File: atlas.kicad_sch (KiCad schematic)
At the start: 26 parts, among them J1 AudioJack3, J2 Micro_SD_Card, SW1 SW_Push, SW2 SW_SPST, SW3 SW_Push, SW4 SW_Push, SW5 SW_Push, SW6 SW_Push, U1 ATmega328-P, U2 DAC8571IDGK, U3 Nokia_5110_LCD, U4 NE5532, Y1 Crystal

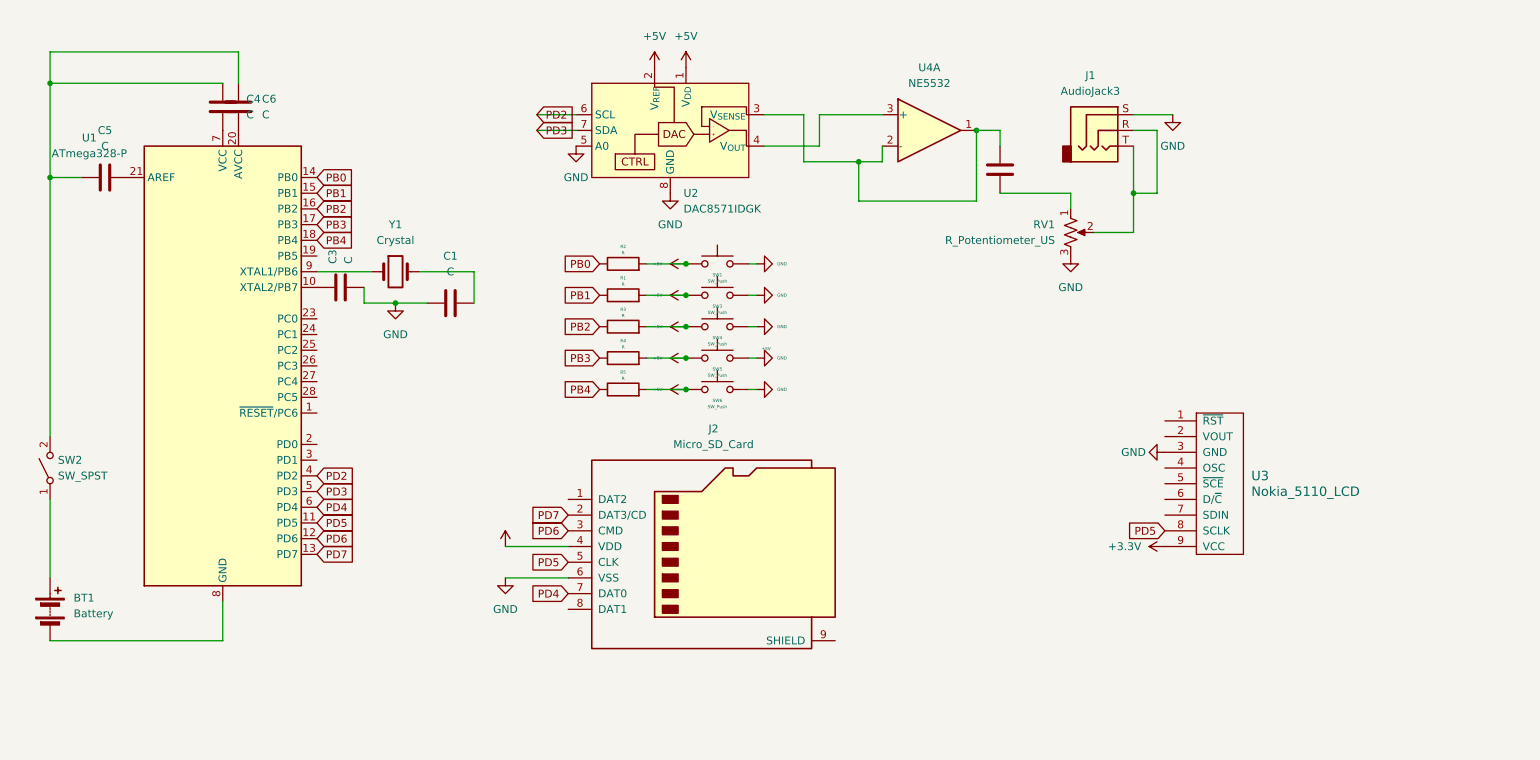
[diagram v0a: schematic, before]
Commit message: Add files via upload
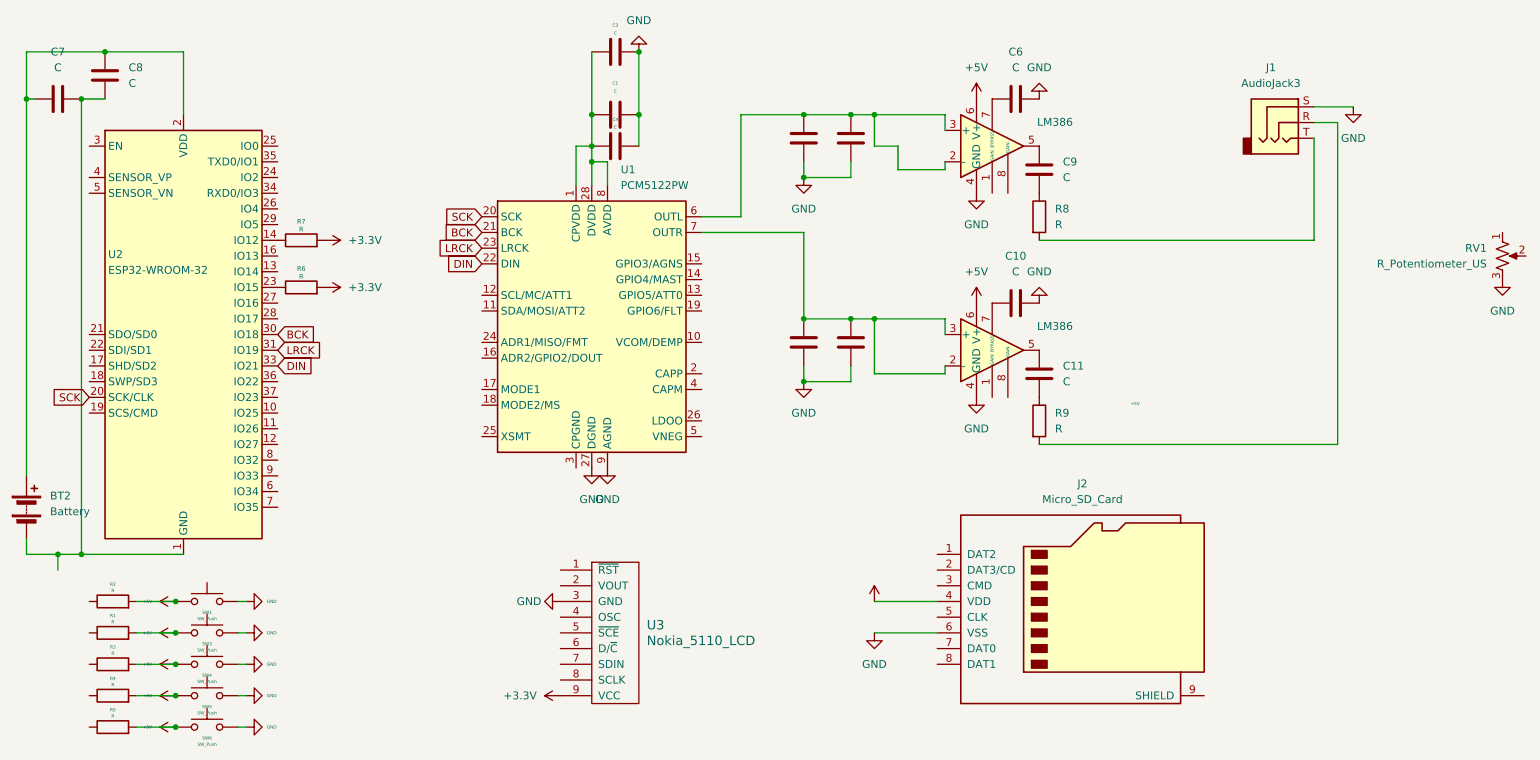
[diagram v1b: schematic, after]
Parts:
- removed BT1: Battery, symbol Device:Battery
- removed SW2: SW_SPST, Button_Switch_THT:SW_PUSH_6mm, symbol Switch:SW_SPST
- removed U1: ATmega328-P, Package_DFN_QFN:HVQFN-32-1EP_5x5mm_P0.5mm_EP3.1x3.1mm, symbol MCU_Microchip_ATmega:ATmega328-P
- removed U2: DAC8571IDGK, Package_SO:MSOP-8_3x3mm_P0.65mm, symbol Analog_DAC:DAC8571IDGK
- removed U4: NE5532, Package_CSP:LFCSP-8_2x2mm_P0.5mm, symbol Amplifier_Operational:NE5532
- removed Y1: Crystal, Crystal:Crystal_C26-LF_D2.1mm_L6.5mm_Horizontal, symbol Device:Crystal
- added BT2: Battery, symbol Device:Battery
- added C10, C11, C12, C13, C7, C8, C9: C, Capacitor_SMD:C_1808_4520Metric_Pad1.72x2.30mm_HandSolder, symbol Device:C
- added R6, R7, R8, R9: R, Resistor_SMD:R_0201_0603Metric, symbol Device:R
- added U1: PCM5122PW, Package_SO:TSSOP-28_4.4x9.7mm_P0.65mm, symbol Audio:PCM5122PW
- added U2: ESP32-WROOM-32, RF_Module:ESP32-WROOM-32, symbol RF_Module:ESP32-WROOM-32
- added U4, U6: LM386, Package_DIP:DIP-8_W7.62mm, symbol Amplifier_Audio:LM386
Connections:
- net +3.3V: now also R6.2, R7.2
- net +5V: now also U4.6 (V+), U6.6 (V+)
- net GND: now also C1.2, C2.2, C4.2, C5.2, C6.2, C10.2, C12.2, C13.2, U1.27 (DGND), U1.9 (AGND), U4.4 (GND), U6.4 (GND); no longer C1.1
- net at C2.1: now also C5.1, U1.6 (OUTL), U6.2 (-), U6.3 (+)
- net at C3.1: now also C1.1, C4.1, U1.1 (CPVDD), U1.28 (DVDD), U1.8 (AVDD)
- net at RV1.1: no longer C2.2
- net PB0: no longer names the net of R2.1
- net PB1: no longer names the net of R1.1
- net PB2: no longer names the net of R3.1
- net PB3: no longer names the net of R4.1
- net PB4: no longer names the net of R5.1
- net PD4: no longer names the net of J2.7 (DAT0)
- net PD5: no longer names the net of U3.8 (SCLK)
- net PD5: no longer J2.5 (CLK)
- net PD6: no longer names the net of J2.3 (CMD)
- net PD7: no longer names the net of J2.2 (DAT3/CD)
- new net: C12.1, C13.1, U1.7 (OUTR), U4.2 (-), U4.3 (+)
- new net: BT2.1 (+), C7.1, C8.1, U2.2 (VDD)
- new net: BT2.2 (-), C7.2, C8.2, U2.1 (GND), U2.15 (GND), U2.38 (GND), U2.39 (GND)
- new net: R7.1, U2.14 (IO12)
- new net: R6.1, U2.23 (IO15)
- new net: C10.1, U4.7 (BYPASS)
- new net: C9.1, U6.5
- new net: C9.2, R8.1
- new net: C6.1, U6.7 (BYPASS)
- new net: J1.R, R9.2
- new net: J1.T, R8.2
- new net: C11.1, U4.5
- new net: C11.2, R9.1
- new net BCK: U1.21 (BCK), U2.30 (IO18)
- new net DIN: U1.22 (DIN), U2.33 (IO21)
- new net LRCK: U1.23 (LRCK), U2.31 (IO19)
- new net SCK: U1.20 (SCK), U2.20 (SCK/CLK)
- now unconnected: RV1.2
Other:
- company: (none) -> Kale
- title: (none) -> Atlas
- moved on the sheet: J1, J2, R1, R2, R3, R4, R5, RV1, SW1, SW3, SW4, SW5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
